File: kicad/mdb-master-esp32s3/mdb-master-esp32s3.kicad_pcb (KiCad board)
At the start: 2 copper layers, 40 x 46 mm, 36 parts, among them J1 Conn_02x11_Odd_Even, J2 USB_C_Receptacle_USB2.0_16P, J3 MDB_Connector, J4 Barrel_Jack, Q1 BC807, SW1 SW_Push, U1 ESP32-S3FH4R2, U2 LM2594HVM-3.3, Y1 Crystal_GND24

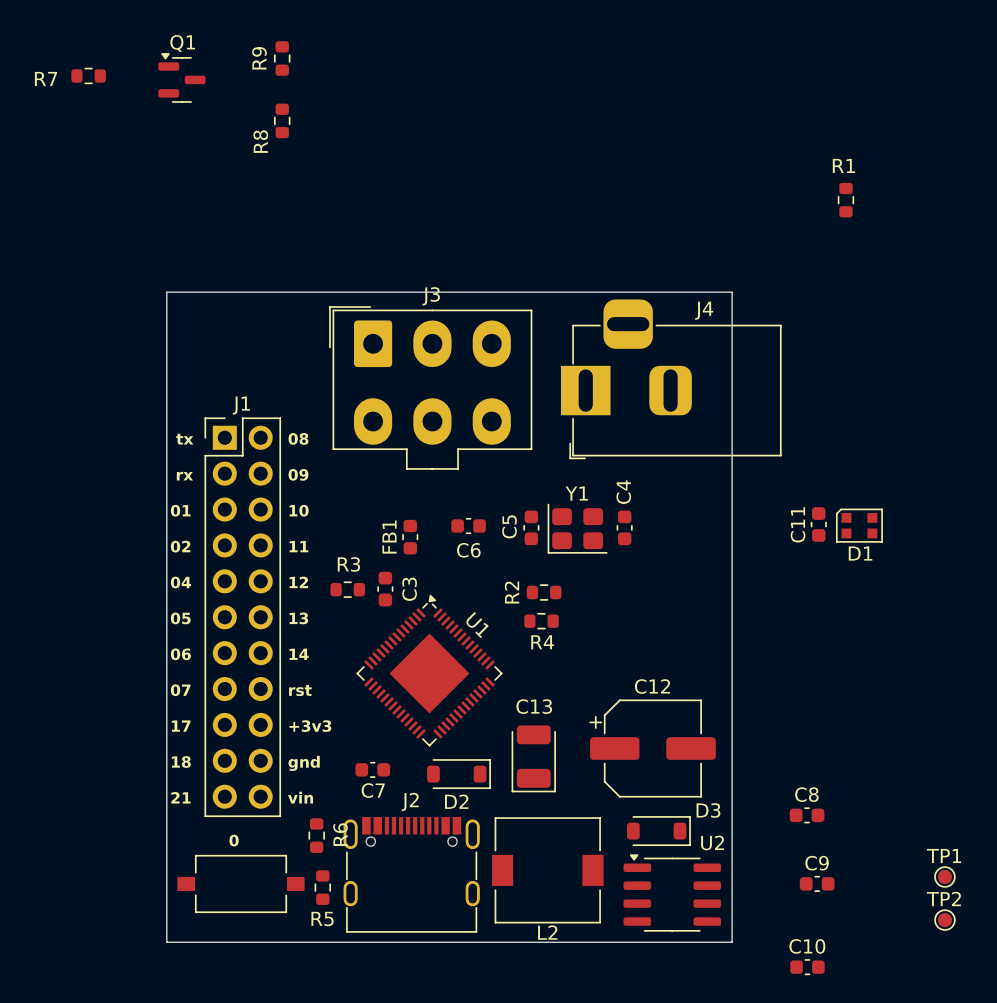
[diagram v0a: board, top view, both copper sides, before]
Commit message: Routing...
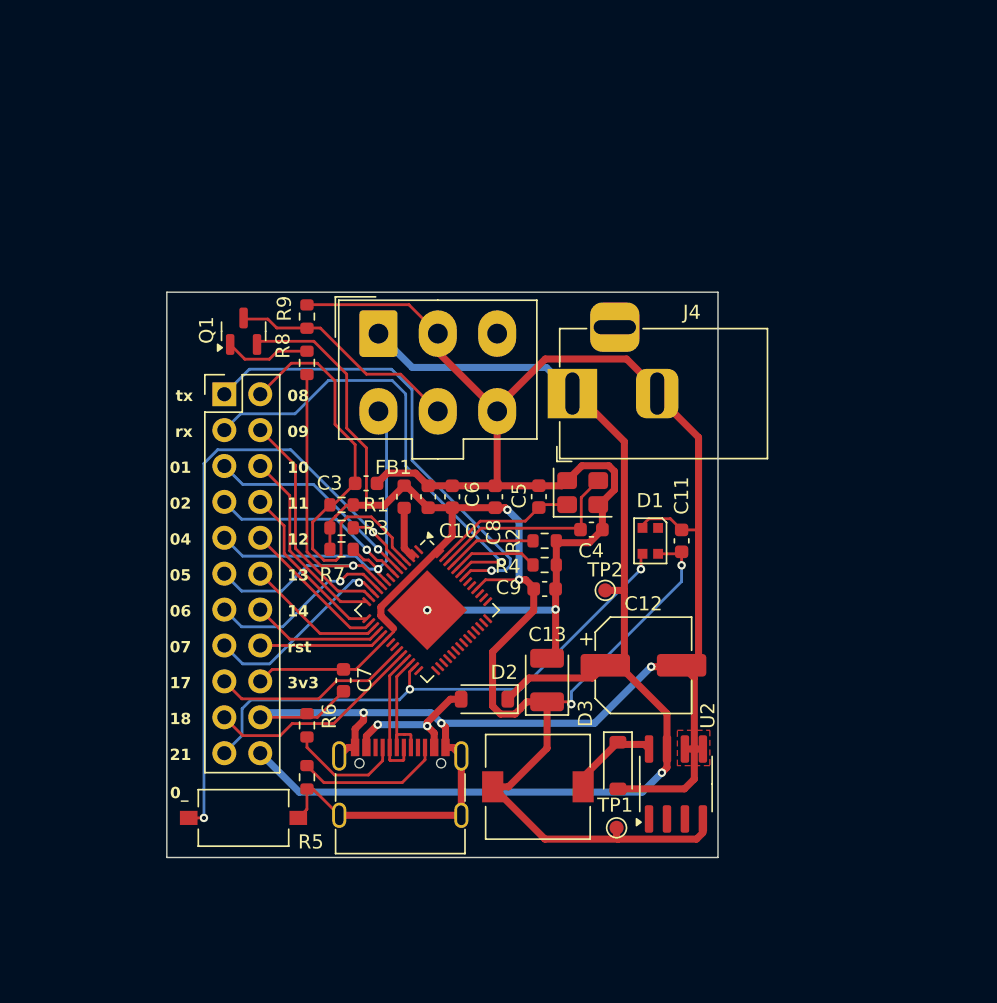
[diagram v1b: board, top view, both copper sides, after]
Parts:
- moved C10 42.8 mm to (144.4, 90.2), turned to -90 degrees
- moved R1 41.7 mm to (138.2, 90.8), turned to 180 degrees
- moved R7 38.0 mm to (138.2, 93.9)
- moved TP2 33.5 mm to (156.9, 96.8)
- moved C8 31.5 mm to (149.1, 90.2), turned to -90 degrees
- moved C9 28.4 mm to (152.6, 96.7), turned to 180 degrees
- moved TP1 23.5 mm to (157.7, 113.6)
- moved R9 18.3 mm to (135.8, 77.4)
- moved Q1 18.3 mm to (131.3, 78.5), turned to 90 degrees
- moved R8 17.2 mm to (135.8, 80.7), turned to 90 degrees
- moved D1 14.8 mm to (160.1, 93.3), turned to -90 degrees
- moved C11 9.77 mm to (162.3, 93.3), turned to -90 degrees
- moved R5 7.88 mm to (135.8, 110.0)
- moved R6 7.84 mm to (135.8, 106.3)
- moved U2 7.83 mm to (161.9, 110.5), turned to 90 degrees
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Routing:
- net GND: track 0.00 -> 187.8 mm, vias 0 -> 5
- net +3V3: track 0.00 -> 123.8 mm, vias 0 -> 4
- net /vin: track 0.00 -> 87.2 mm, vias 0 -> 1
- net /boot: track 0.00 -> 45.7 mm, vias 0 -> 2
- net /io21: track 0.00 -> 38.9 mm, vias 0 -> 2
- net /u0txd: track 0.00 -> 33.6 mm, vias 0 -> 1
- net /u0rxd: track 0.00 -> 32.7 mm, vias 0 -> 1
- net /reset: track 0.00 -> 31.9 mm
- net /io5: track 0.00 -> 29.3 mm, vias 0 -> 1
- net /io4: track 0.00 -> 26.9 mm, vias 0 -> 1
- net /mdb_master_transmit: track 0.00 -> 16.5 mm
- net /io8: track 0.00 -> 16.2 mm
- net /io18: track 0.00 -> 15.5 mm
- net /io1: track 0.00 -> 15.4 mm, vias 0 -> 1
- net Net-(U1-XTAL_N): track 0.00 -> 14.6 mm
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- added copper zone on F.Cu, net GND
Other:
- board size 40 x 46 mm -> 39 x 40 mm
- board text added: "0_"
- board text added: "3v3"
- board text removed: "+3v3"
- board text removed: "0"

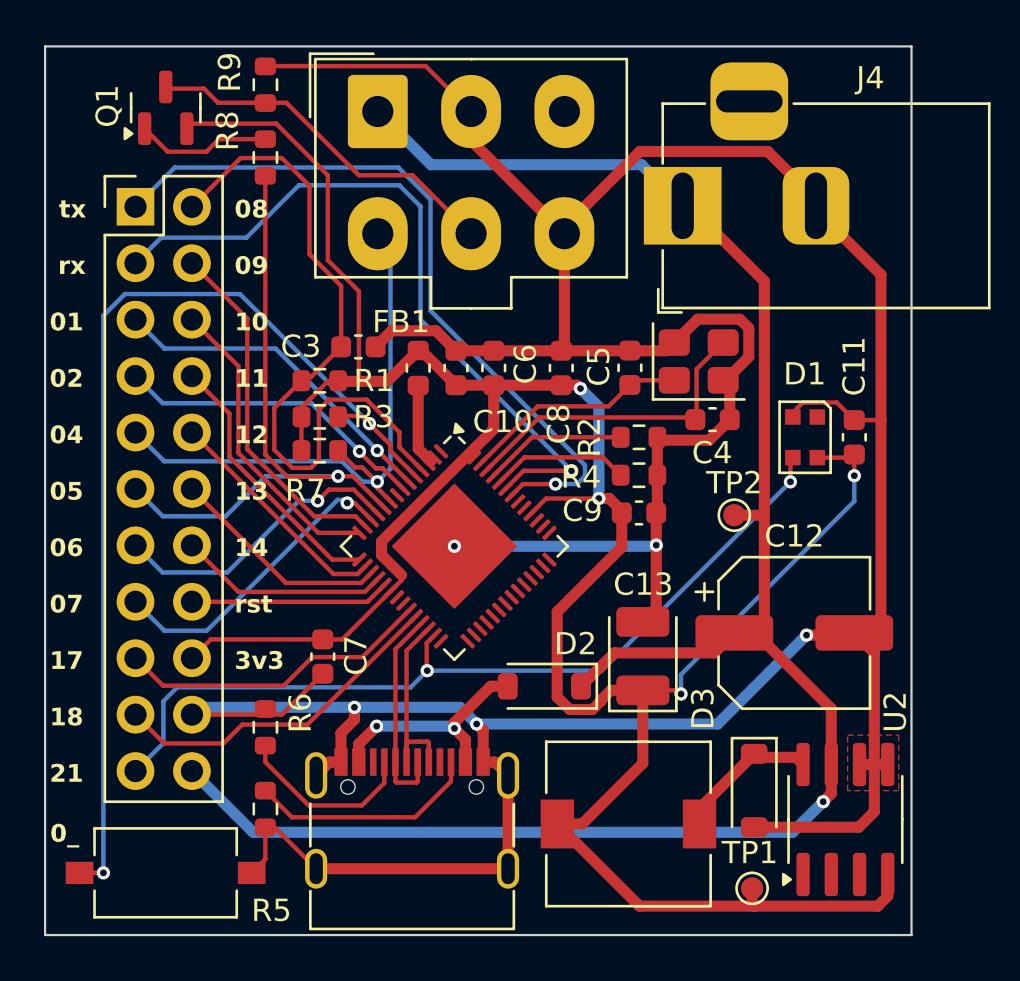
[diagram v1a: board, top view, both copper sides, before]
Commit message: Routing
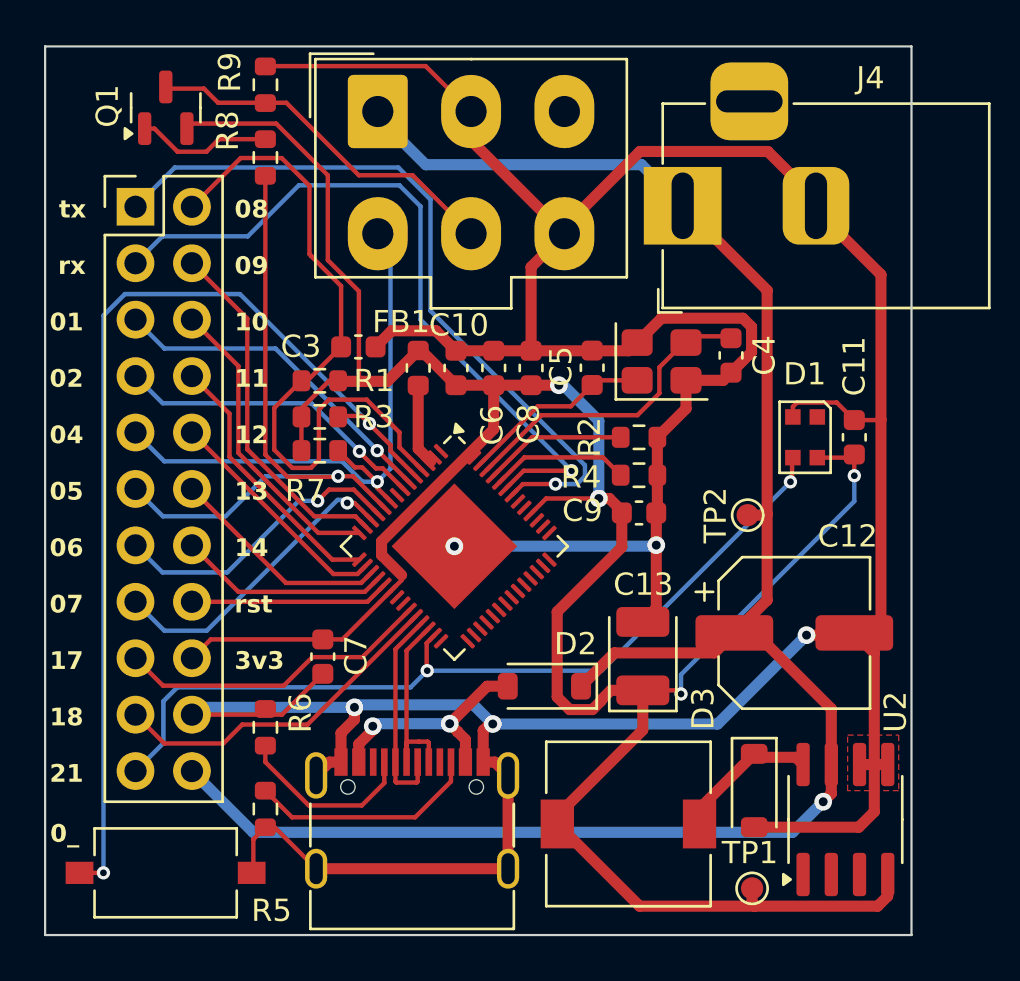
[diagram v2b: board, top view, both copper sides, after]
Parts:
- added REF**: OSHW-Logo2_14.6x12mm_SilkScreen, Symbol:OSHW-Logo2_14.6x12mm_SilkScreen, B.Cu at (156.0, 107.0)
- moved C4 3.01 mm to (156.8, 89.6), turned to 90 degrees
- moved C5 1.70 mm to (150.5, 90.2)
- moved Y1 1.68 mm to (153.6, 89.9)
- moved C8 1.36 mm to (147.8, 90.2)
- moved TP2 0.60 mm to (157.5, 96.8), turned to 90 degrees
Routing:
- net Net-(U1-XTAL_P): track 10.3 -> 8.62 mm
- net /vin: track 87.2 -> 86.1 mm
- net +3V3: track 123.8 -> 122.8 mm
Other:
- board text added: "VMflow.xyz"
- board text added: "mdb-controller-esp32s3"
- board text removed: "mdb-master-esp32s3"
